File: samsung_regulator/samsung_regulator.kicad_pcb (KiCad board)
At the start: 2 copper layers, 9 parts, among them K1 CONN_3

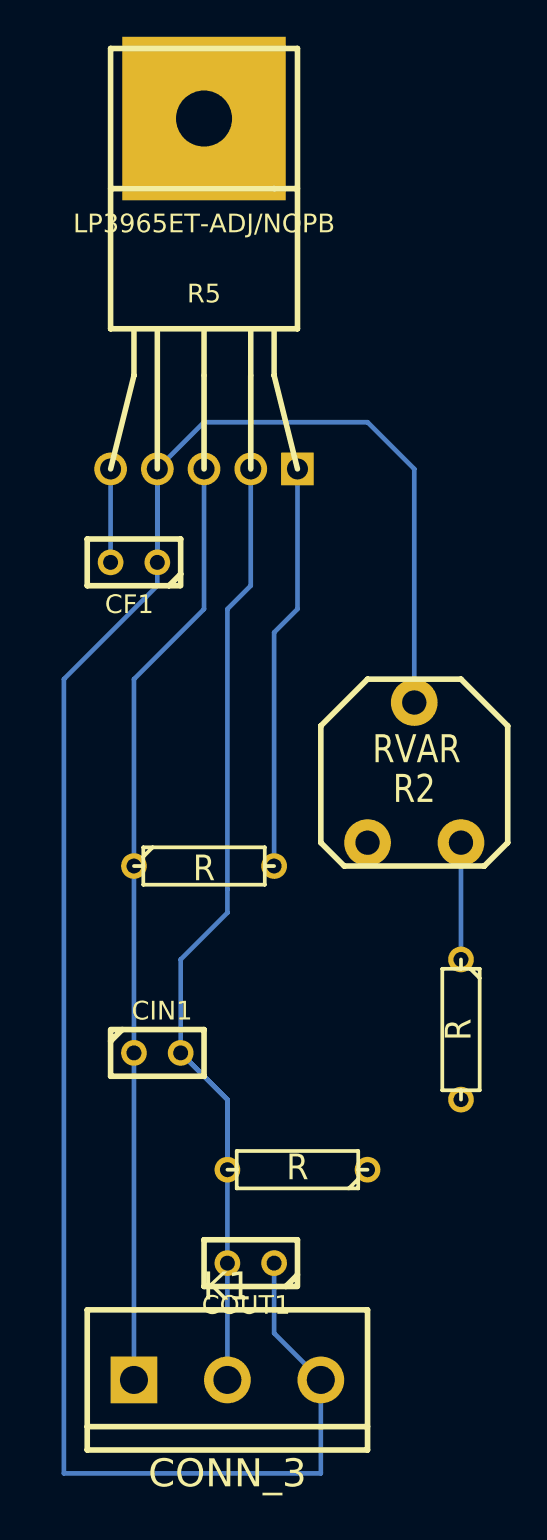
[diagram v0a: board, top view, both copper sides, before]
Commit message: connected all
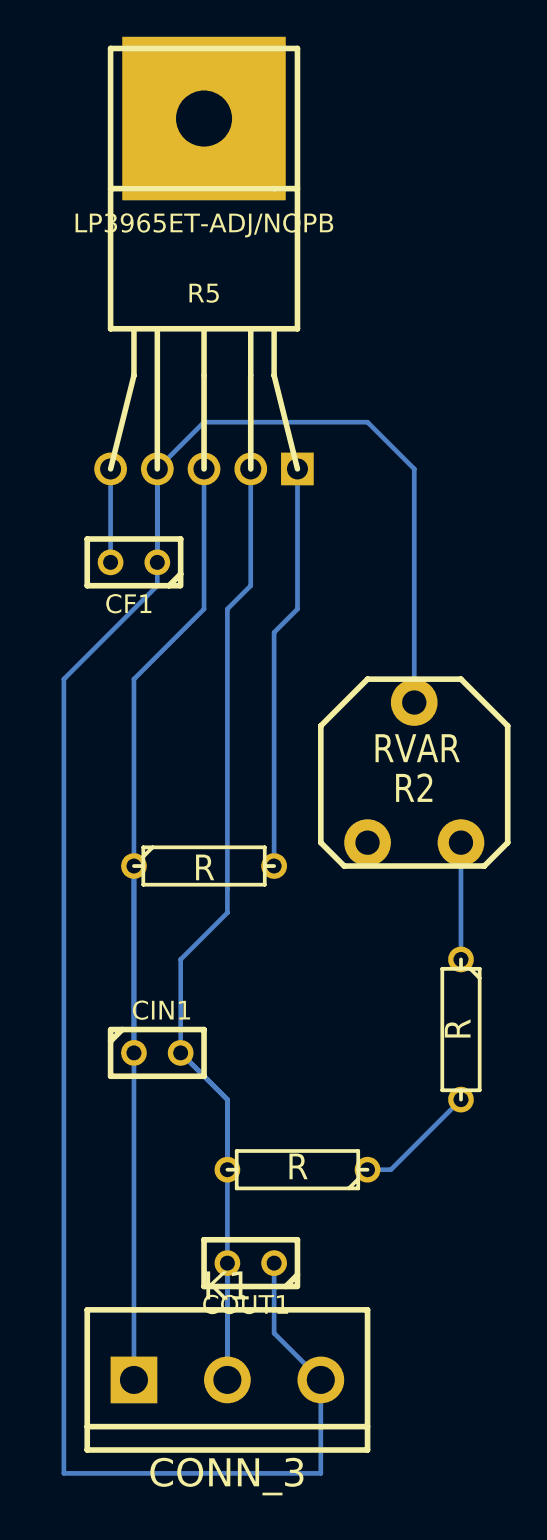
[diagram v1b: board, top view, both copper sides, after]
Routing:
- net N-000007: track 51.1 -> 61.3 mm
- net N-000005: track 0.00 -> 6.66 mm
- net GND: track 59.6 -> 65.9 mm
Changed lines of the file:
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@@
   (general
     (links 15)
-    (no_connects 3)
+    (no_connects 0)
     (area 175.468845 42.98982 202.336401 124.3584)
     (thickness 1.6)
     (drawings 0)
-    (tracks 34)
+    (tracks 38)
     (zones 0)
     (modules 9)
@@
     )
   )
+  (segment (start 186.69 118.11) (end 186.69 111.76) (width 0.254) (layer B.Cu) (net 1))
   (segment (start 186.69 106.68) (end 186.69 102.87) (width 0.254) (layer B.Cu) (net 1))
   (segment (start 186.69 102.87) (end 184.15 100.33) (width 0.254) (layer B.Cu) (net 1))
@@
   (segment (start 189.23 77.47) (end 190.5 76.2) (width 0.254) (layer B.Cu) (net 3))
   (segment (start 199.39 95.25) (end 199.39 88.9) (width 0.254) (layer B.Cu) (net 4))
+  (segment (start 194.31 106.68) (end 195.58 106.68) (width 0.254) (layer B.Cu) (net 5))
+  (segment (start 195.58 106.68) (end 199.39 102.87) (width 0.254) (layer B.Cu) (net 5))
   (segment (start 196.85 81.28) (end 196.85 68.58) (width 0.254) (layer B.Cu) (net 6))
   (segment (start 185.42 66.04) (end 182.88 68.58) (width 0.254) (layer B.Cu) (net 6))
@@
   (segment (start 177.8 123.19) (end 177.8 80.01) (width 0.254) (layer B.Cu) (net 6))
   (segment (start 191.77 123.19) (end 177.8 123.19) (width 0.254) (layer B.Cu) (net 6))
+  (segment (start 181.61 100.33) (end 181.61 90.17) (width 0.254) (layer B.Cu) (net 7))
   (segment (start 181.61 118.11) (end 181.61 100.33) (width 0.254) (layer B.Cu) (net 7))
   (segment (start 181.61 100.33) (end 181.61 80.01) (width 0.254) (layer B.Cu) (net 7))
